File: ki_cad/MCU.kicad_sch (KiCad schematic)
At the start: 13 parts, among them J11 SWD_CONN, SW1 USER_SW, U1 STM32L010F4P6

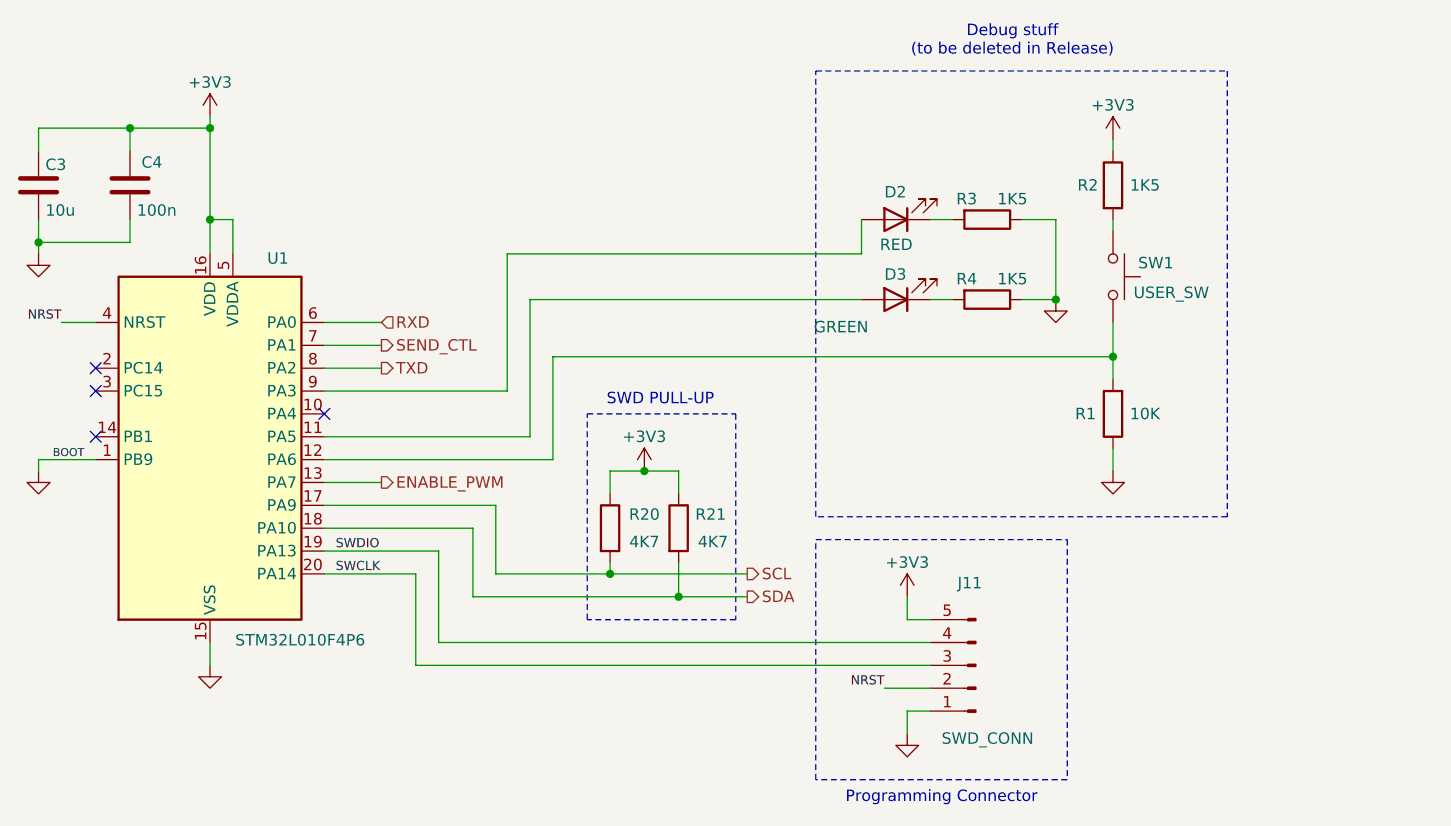
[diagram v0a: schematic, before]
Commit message: update parts && add test points
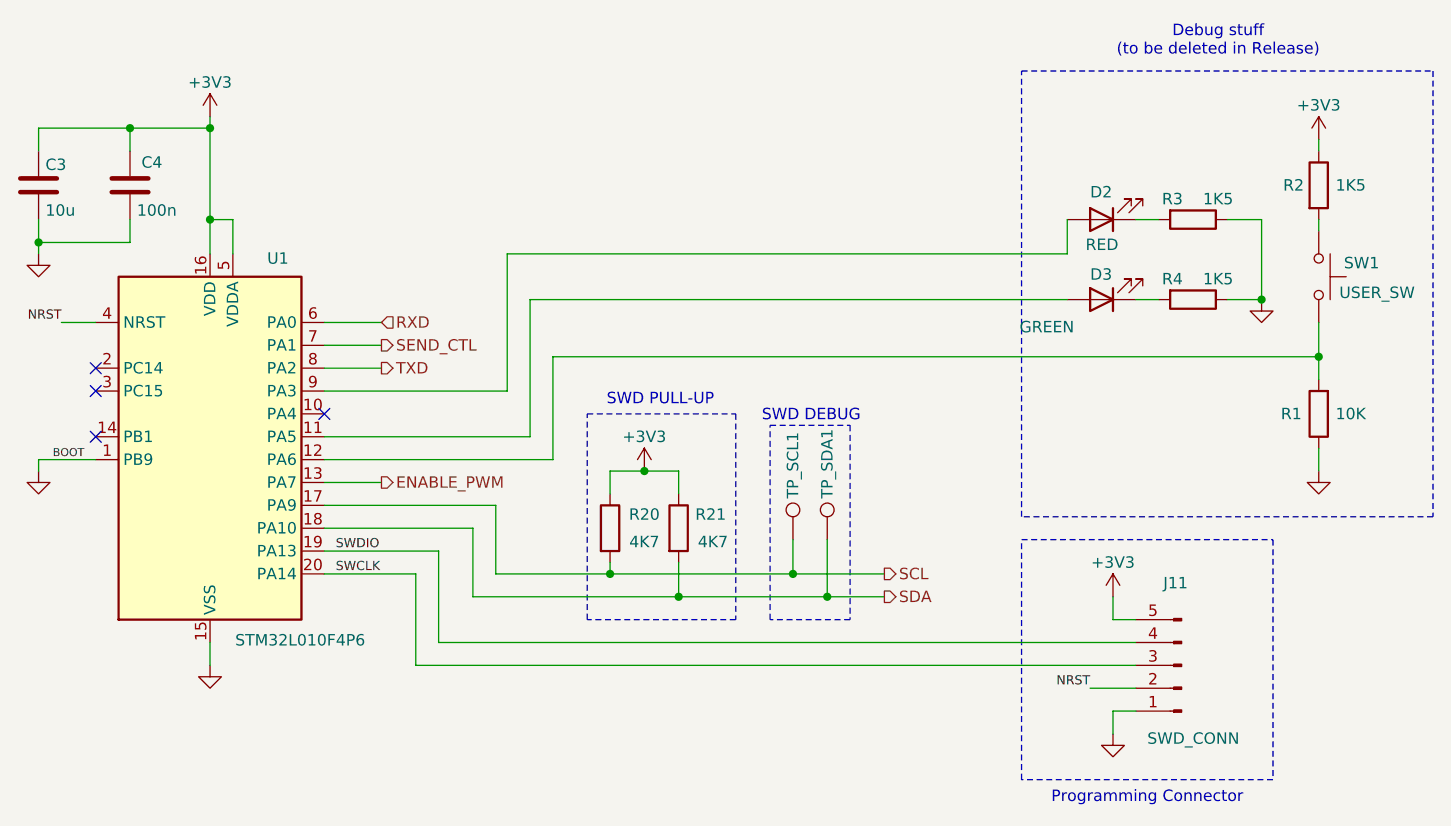
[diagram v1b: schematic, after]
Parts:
- added TP_SCL1, TP_SDA1: TestPoint, TestPoint:TestPoint_Pad_D1.5mm, symbol Connector:TestPoint
- R2, R3, R4: footprint Resistor_SMD:R_0201_0603Metric -> Resistor_SMD:R_0402_1005Metric; JLCPCB Part # C22843 -> C25867
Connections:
- net SCL: now also TP_SCL1.1
- net SDA: now also TP_SDA1.1
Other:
- note added: "SWD DEBUG"
- moved on the sheet: D2, D3, J11, R1, R2, R3, R4, SW1

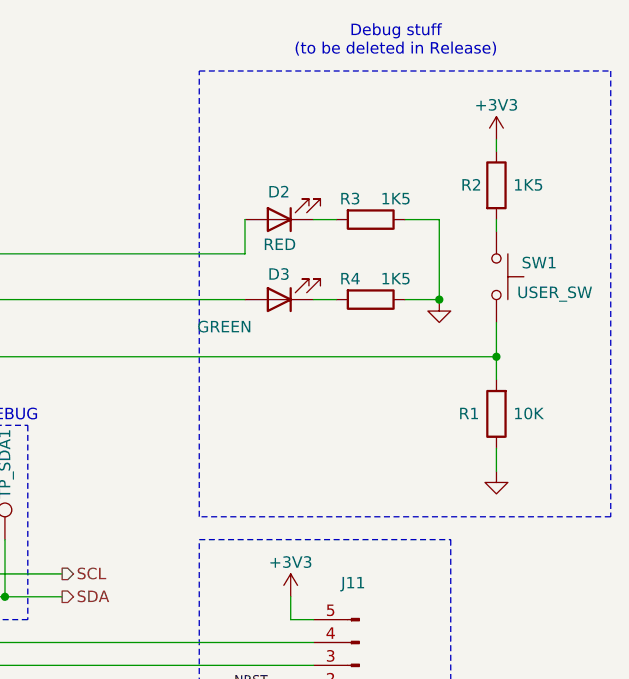
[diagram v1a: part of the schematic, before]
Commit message: update code
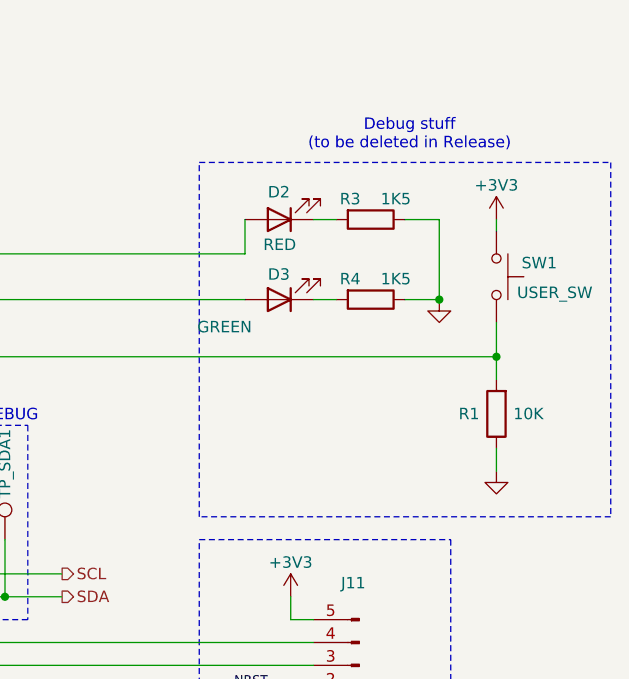
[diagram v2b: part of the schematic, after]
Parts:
- removed R2: 1K5, Resistor_SMD:R_0402_1005Metric, symbol Device:R
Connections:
- net +3V3: now also SW1.1
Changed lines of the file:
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@@
 	)
 	(rectangle
-		(start 144.78 20.32)
+		(start 144.78 30.48)
 		(end 190.5 69.85)
 		(stroke
@@
 	(text "Debug stuff\n(to be deleted in Release)"
 		(exclude_from_sim no)
-		(at 166.624 17.018 0)
+		(at 168.148 27.432 0)
 		(effects
 			(font
@@
 	(no_connect
 		(at 41.91 60.96)
-	)
-	(wire
-		(pts
-			(xy 177.8 27.94) (xy 177.8 29.21)
-		)
-		(stroke
-			(width 0)
-			(type default)
-		)
 	)
 	(wire
@@
 		)
 		(instances
-			(project ""
+			(project "pwm_board"
 				(path "/71ddf0e9-b3bd-413d-a31e-e27757e0e466/7c9a574e-1626-44f3-9594-09b30c5119d2"
 					(reference "SW1")
@@
 		)
 		(instances
-			(project ""
+			(project "pwm_board"
 				(path "/71ddf0e9-b3bd-413d-a31e-e27757e0e466/7c9a574e-1626-44f3-9594-09b30c5119d2"
 					(reference "U1")
@@
 		)
 		(instances
-			(project ""
+			(project "pwm_board"
 				(path "/71ddf0e9-b3bd-413d-a31e-e27757e0e466/7c9a574e-1626-44f3-9594-09b30c5119d2"
 					(reference "TP_SCL1")
@@
 	(symbol
 		(lib_id "power:+3V3")
-		(at 177.8 27.94 0)
+		(at 177.8 36.83 0)
 		(unit 1)
 		(exclude_from_sim no)
@@
 		(dnp no)
 		(property "Reference" "#PWR010"
-			(at 177.8 31.75 0)
+			(at 177.8 40.64 0)
 			(effects
 				(font
@@
 		)
 		(property "Value" "+3V3"
-			(at 177.8 24.13 0)
+			(at 177.8 33.02 0)
 			(effects
 				(font
@@
 		)
 		(property "Footprint" ""
-			(at 177.8 27.94 0)
+			(at 177.8 36.83 0)
 			(effects
 				(font
@@
 		)
 		(property "Datasheet" ""
-			(at 177.8 27.94 0)
+			(at 177.8 36.83 0)
 			(effects
 				(font
@@
 		)
 		(property "Description" "Power symbol creates a global label with name \"+3V3\""
-			(at 177.8 27.94 0)
+			(at 177.8 36.83 0)
 			(effects
 				(font
@@
 		)
 		(instances
-			(project ""
+			(project "pwm_board"
 				(path "/71ddf0e9-b3bd-413d-a31e-e27757e0e466/7c9a574e-1626-44f3-9594-09b30c5119d2"
 					(reference "J11")
 					(unit 1)
 				)
-			)
-		)
-	)
-	(symbol
-		(lib_id "Device:R")
-		(at 177.8 33.02 0)
-		(unit 1)
-		(exclude_from_sim no)
-		(in_bom yes)
-		(on_board yes)
-		(dnp no)
-		(property "Reference" "R2"
-			(at 175.006 33.02 0)
-			(effects
-				(font
-					(size 1.27 1.27)
-				)
-			)
-		)
-		(property "Value" "1K5"
-			(at 181.356 33.02 0)
-			(effects
-				(font
-					(size 1.27 1.27)
-				)
-			)
-		)
-		(property "Footprint" "Resistor_SMD:R_0402_1005Metric"
-			(at 176.022 33.02 90)
-			(effects
-				(font
-					(size 1.27 1.27)
-				)
-				(hide yes)
-			)
-		)
-		(property "Datasheet" "~"
-			(at 177.8 33.02 0)
-			(effects
-				(font
-					(size 1.27 1.27)
-				)
-				(hide yes)
-			)
-		)
-		(property "Description" "Resistor"
-			(at 177.8 33.02 0)
-			(effects
-				(font
-					(size 1.27 1.27)
-				)
-				(hide yes)
-			)
-		)
-		(property "JLCPCB Part #" "C25867"
-			(at 177.8 33.02 90)
-			(effects
-				(font
-					(size 1.27 1.27)
-				)
-				(hide yes)
-			)
-		)
-		(property "KLC_S3.3" ""
-			(at 177.8 33.02 90)
-			(effects
-				(font
-					(size 1.27 1.27)
-				)
-				(hide yes)
-			)
-		)
-		(property "KLC_S4.1" ""
-			(at 177.8 33.02 90)
-			(effects
-				(font
-					(size 1.27 1.27)
-				)
-				(hide yes)
-			)
-		)
-		(property "Sim.Device" ""
-			(at 177.8 33.02 90)
-			(effects
-				(font
-					(size 1.27 1.27)
-				)
-				(hide yes)
-			)
-		)
-		(property "Sim.Type" ""
-			(at 177.8 33.02 90)
-			(effects
-				(font
-					(size 1.27 1.27)
-				)
-				(hide yes)
-			)
-		)
-		(property "Field9" ""
-			(at 177.8 33.02 0)
-			(effects
-				(font
-					(size 1.27 1.27)
-				)
-				(hide yes)
-			)
-		)
-		(pin "2"
-		)
-		(pin "1"
-		)
-		(instances
-			(project "pwm_board"
-				(path "/71ddf0e9-b3bd-413d-a31e-e27757e0e466/7c9a574e-1626-44f3-9594-09b30c5119d2"
-					(reference "R2")
-					(unit 1)
-				)
